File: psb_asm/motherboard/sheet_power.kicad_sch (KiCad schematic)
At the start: 3 parts, among them J1 Conn_01x10_Socket, J2 Conn_01x10_Socket, U12 LD1117S12TR_SOT223

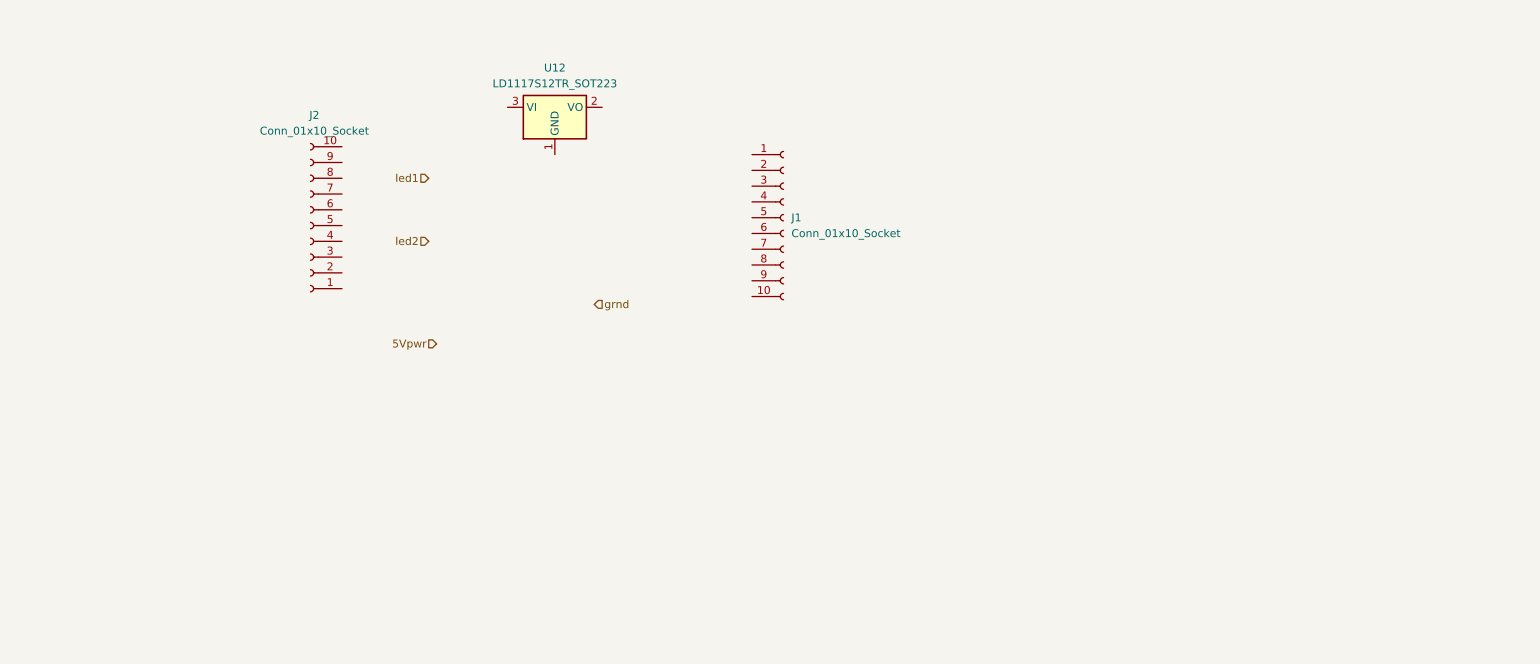
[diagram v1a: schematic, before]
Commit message: motherboard_power
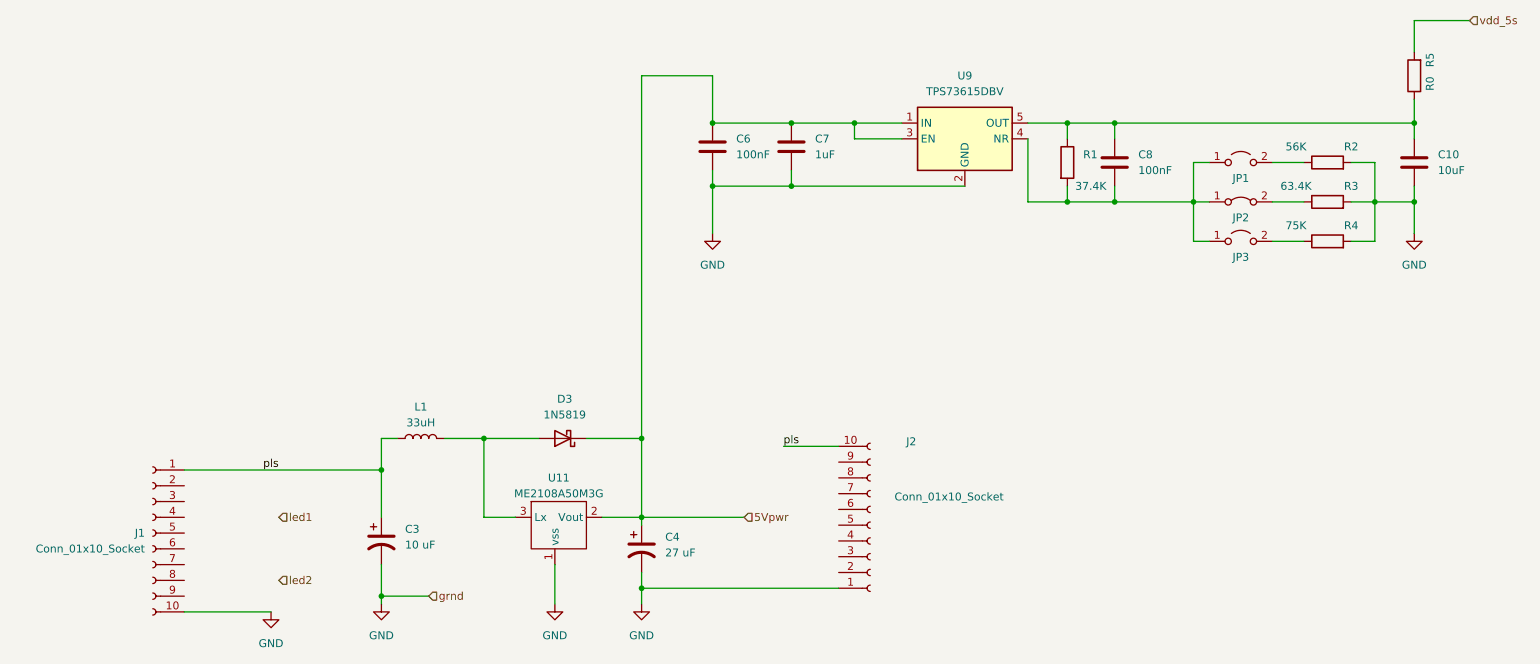
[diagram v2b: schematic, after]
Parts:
- removed U12: LD1117S12TR_SOT223, Package_TO_SOT_SMD:SOT-223-3_TabPin2, symbol Regulator_Linear:LD1117S12TR_SOT223
- added C10: 10uF, Capacitor_Tantalum_SMD:CP_EIA-1608-08_AVX-J, symbol Device:C
- added C3: 10 uF, symbol Device:C_Polarized_US
- added C4: 27 uF, symbol Device:C_Polarized_US
- added C6, C8: 100nF, Capacitor_Tantalum_SMD:CP_EIA-1608-08_AVX-J, symbol Device:C
- added C7: 1uF, Capacitor_Tantalum_SMD:CP_EIA-1608-08_AVX-J, symbol Device:C
- added D3: 1N5819, symbol Device:D_Schottky
- added JP1, JP3: Jumper_2_Open, mouse:jump_off, symbol Jumper:Jumper_2_Open
- added JP2: Jumper_2_Bridged, mouse:Jump_on, symbol Jumper:Jumper_2_Bridged
- added L1: 33uH, symbol Device:L
- added R1: 37.4K, Resistor_SMD:R_0603_1608Metric, symbol Device:R
- added R2: 56K, Resistor_SMD:R_0603_1608Metric, symbol Device:R
- added R3: 63.4K, Resistor_SMD:R_0603_1608Metric, symbol Device:R
- added R4: 75K, Resistor_SMD:R_0603_1608Metric, symbol Device:R
- added R5: R0, Resistor_SMD:R_0603_1608Metric, symbol Device:R
- added U11: ME2108A50M3G, Package_TO_SOT_SMD:SOT-23, symbol pwr_supply01:ME2108A50M3G
- added U9: TPS73615DBV, Package_TO_SOT_SMD:SOT-23-5, symbol Regulator_Linear:TPS73615DBV
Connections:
- net 5Vpwr: now also C4.1, C6.1, C7.1, D3.1 (K), U11.2 (Vout), U9.1 (IN), U9.3 (EN)
- net GND: now reaches J2.1 (Pin_1)
- net GND: now also J1.10 (Pin_10), C10.2, C3.2, C4.2, C6.2, C7.2, R2.2, R3.2, R4.2, U11.1 (vss), U9.2 (GND)
- net pls: now reaches J2.10 (Pin_10)
- net pls: now also J1.1 (Pin_1), C3.1, L1.1
- new net: D3.2 (A), L1.2, U11.3 (Lx)
- new net: JP1.2 (B), R2.1
- new net: JP3.2 (B), R4.1
- new net: C10.1, C8.1, R1.1, R5.1, U9.5 (OUT)
- new net: C8.2, JP1.1 (A), JP2.1 (A), JP3.1 (A), R1.2, U9.4 (NR)
- new net: JP2.2 (B), R3.1
- new net vdd_5s: R5.2
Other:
- moved on the sheet: J1, J2
